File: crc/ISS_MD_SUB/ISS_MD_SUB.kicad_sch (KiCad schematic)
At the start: 3 parts, among them J1 Conn_01x06, SW1 SW_MEC_5E, U1 STM32F303K8Tx

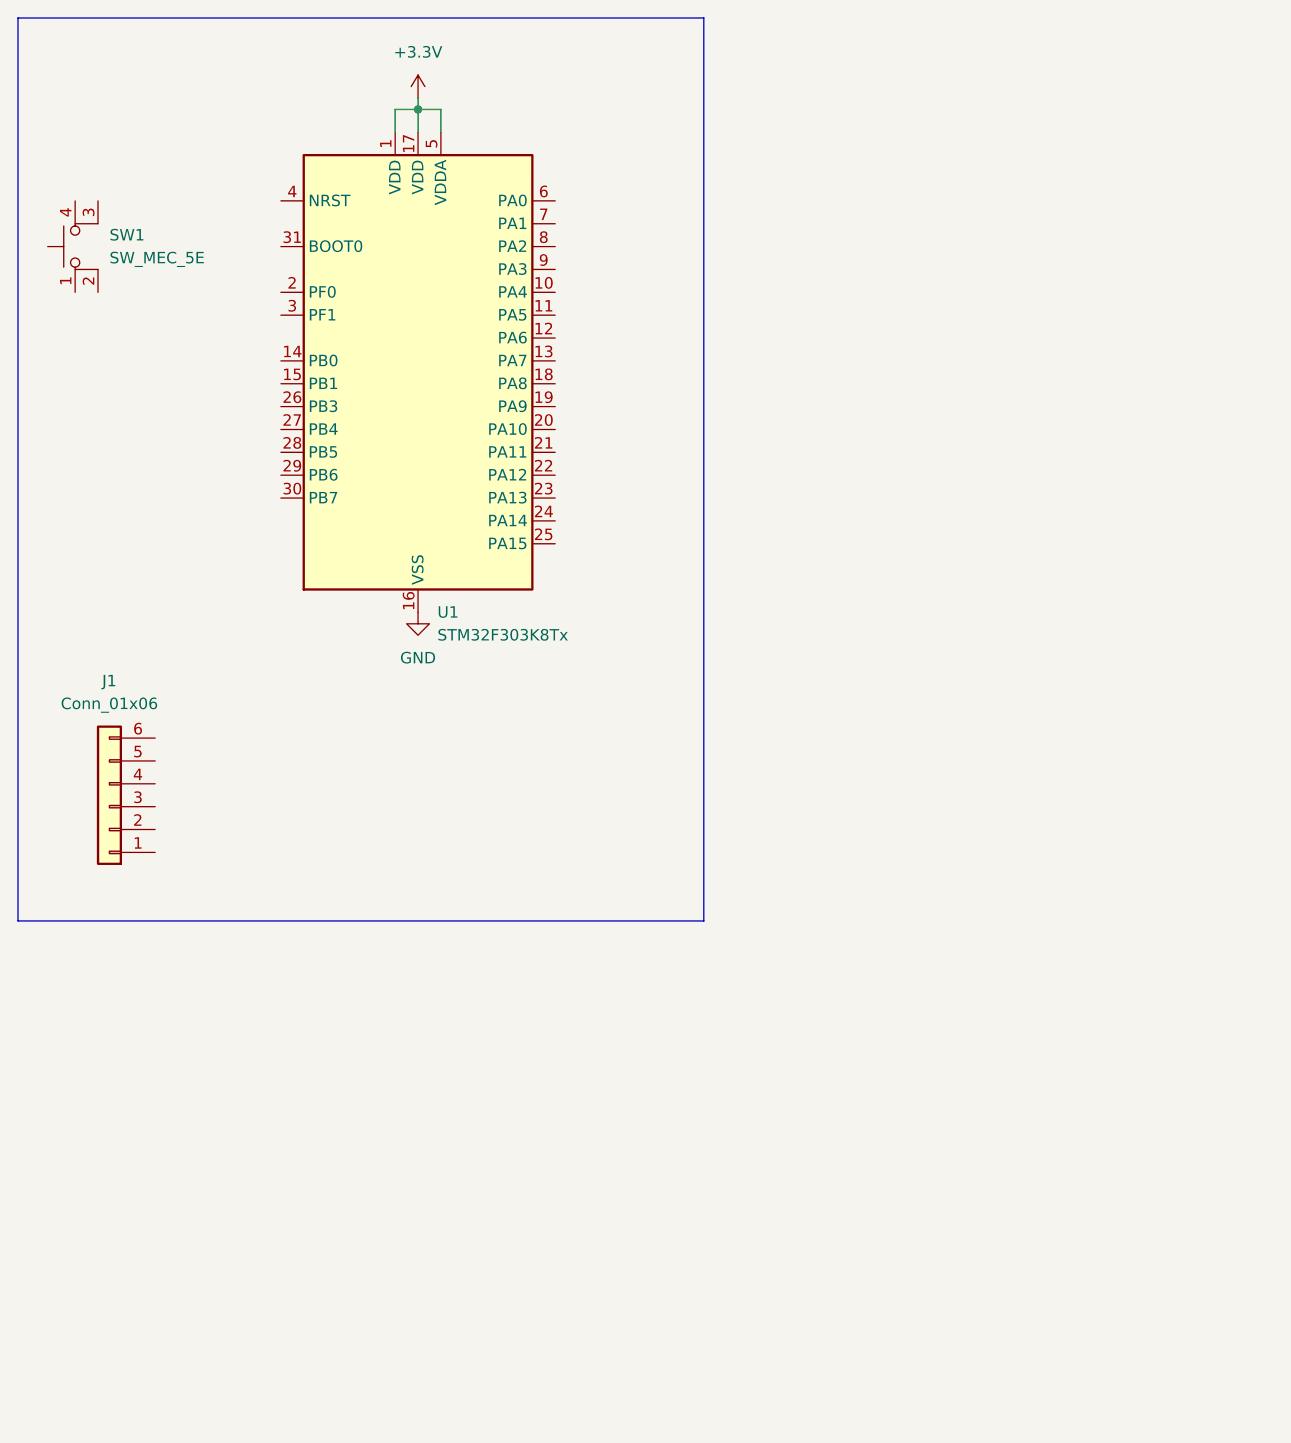
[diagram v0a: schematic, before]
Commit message: 基板2枚め
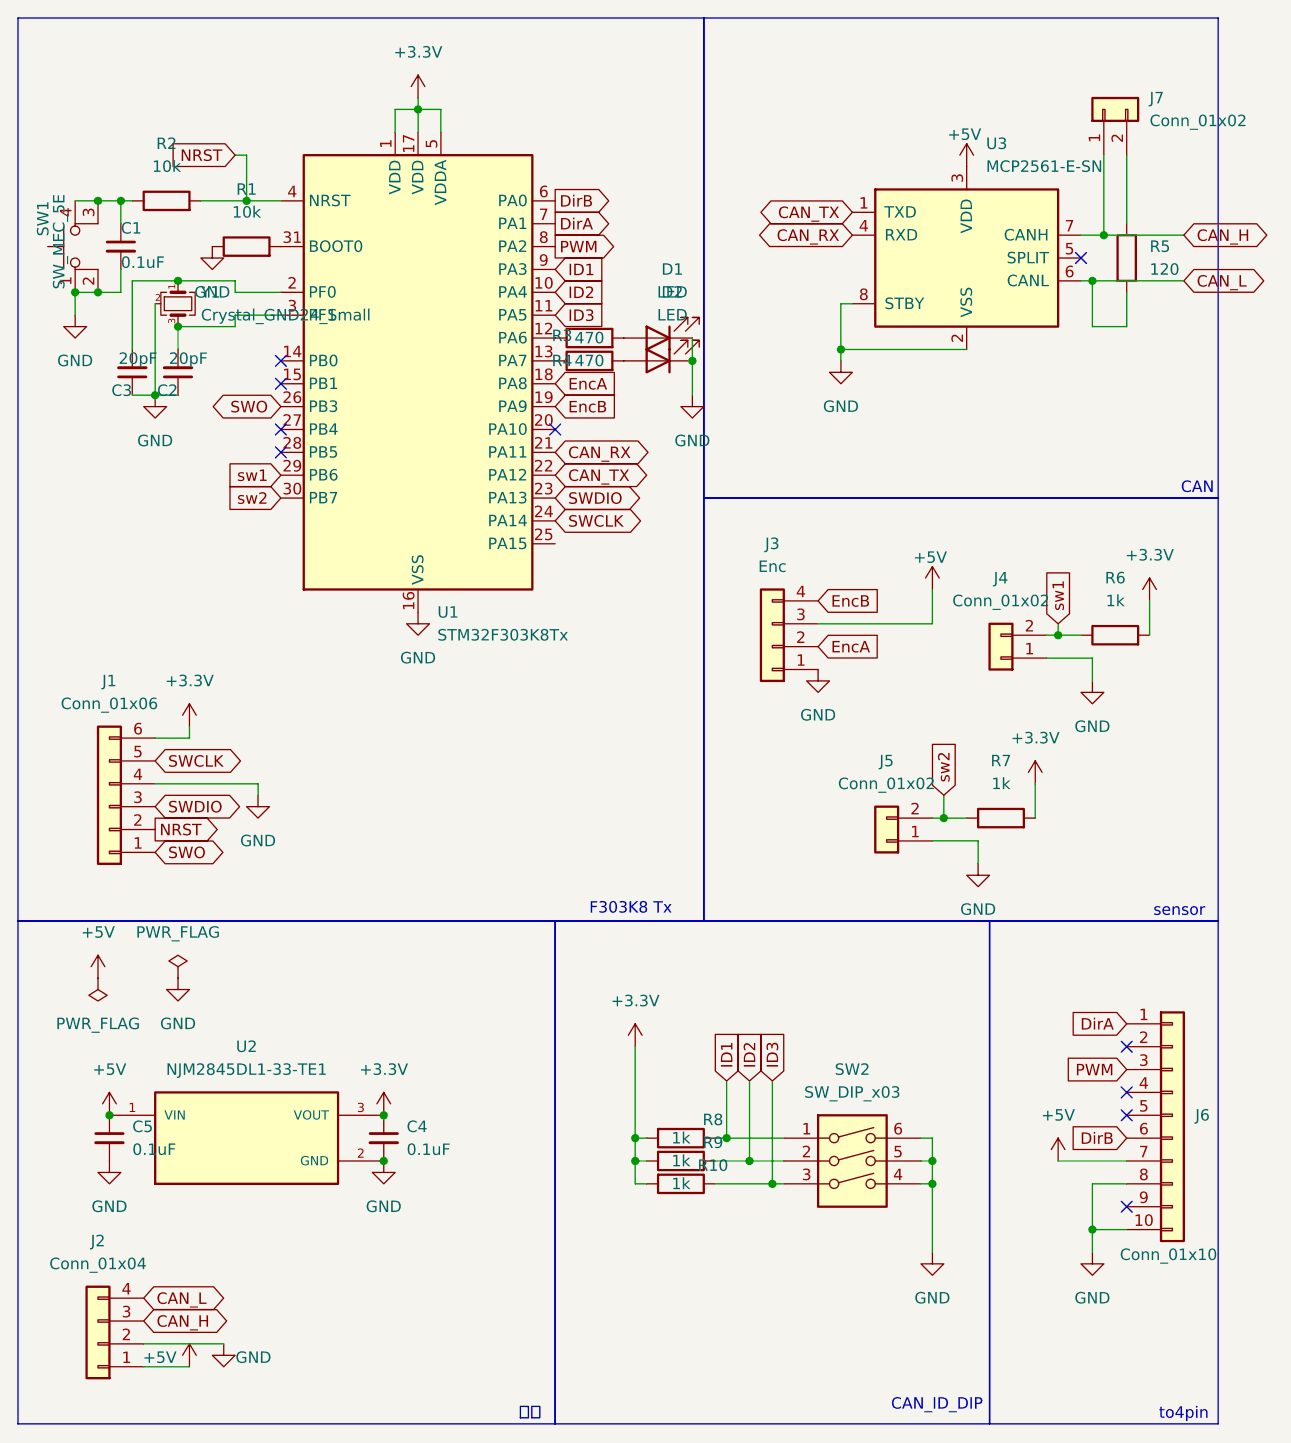
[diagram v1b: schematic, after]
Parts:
- added C1, C4, C5: 0.1uF, Capacitor_SMD:C_0603_1608Metric_Pad1.08x0.95mm_HandSolder, symbol Device:C_Small
- added C2, C3: 20pF, Capacitor_SMD:C_0603_1608Metric_Pad1.08x0.95mm_HandSolder, symbol Device:C_Small
- added D1, D2: LED, LED_SMD:LED_0603_1608Metric_Pad1.05x0.95mm_HandSolder, symbol Device:LED
- added J2: Conn_01x04, Connector_JST:JST_XH_S4B-XH-A_1x04_P2.50mm_Horizontal, symbol Connector_Generic:Conn_01x04
- added J3: Enc, Connector_JST:JST_XH_S4B-XH-A_1x04_P2.50mm_Horizontal, symbol Connector_Generic:Conn_01x04
- added J4, J5: Conn_01x02, Connector_JST:JST_XH_B2B-XH-A_1x02_P2.50mm_Vertical, symbol Connector_Generic:Conn_01x02
- added J6: Conn_01x10, Connector_PinSocket_2.54mm:PinSocket_1x10_P2.54mm_Vertical, symbol Connector_Generic:Conn_01x10
- added J7: Conn_01x02, Connector_PinHeader_2.54mm:PinHeader_1x02_P2.54mm_Vertical, symbol Connector_Generic:Conn_01x02
- added R1, R2: 10k, Resistor_SMD:R_0603_1608Metric_Pad0.98x0.95mm_HandSolder, symbol Device:R
- added R10, R6, R7, R8, R9: 1k, Resistor_SMD:R_0603_1608Metric_Pad0.98x0.95mm_HandSolder, symbol Device:R
- added R3, R4: 470, Resistor_SMD:R_0603_1608Metric_Pad0.98x0.95mm_HandSolder, symbol Device:R
- added R5: 120, Resistor_SMD:R_0603_1608Metric_Pad0.98x0.95mm_HandSolder, symbol Device:R
- added SW2: SW_DIP_x03, Button_Switch_SMD:SW_DIP_SPSTx03_Slide_6.7x9.18mm_W6.73mm_P2.54mm_LowProfile_JPin, symbol Switch:SW_DIP_x03
- added U2: NJM2845DL1-33-TE1, NJM2845DL1-33-TE1:DPAK228P968X238-4N, symbol NJM2845DL1-33-TE1:NJM2845DL1-33-TE1
- added U3: MCP2561-E-SN, Package_SO:SOIC-8_3.9x4.9mm_P1.27mm, symbol Interface_CAN_LIN:MCP2561-E-SN
- added Y1: Crystal_GND24_Small, TSX_3225_25_0000MF10P_C0:XTAL_TSX-3225_25.0000MF10P-C0, symbol Device:Crystal_GND24_Small
- J1: footprint (none) -> Connector_PinHeader_2.54mm:PinHeader_1x06_P2.54mm_Vertical
- SW1: footprint (none) -> SKRPABE010:SW4_SKRPABE010_ALPS
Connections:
- net +3.3V: now also J1.6 (Pin_6), C4.1, R10.2, R6.2, R7.2, R8.2, R9.2, U2.3 (VOUT)
- net GND: now also J1.4 (Pin_4), SW1.1, SW1.2, C1.2, C2.1, C3.1, C4.2, C5.2, D1.1 (K), D2.1 (K), J2.2 (Pin_2), J3.1 (Pin_1), J4.1 (Pin_1), J5.1 (Pin_1), J6.10 (Pin_10), J6.8 (Pin_8), R1.1, SW2.4, SW2.5, SW2.6, U2.2 (GND), U3.2 (VSS), U3.8 (STBY), Y1.2 (G), Y1.4 (G)
- net SWO: now reaches J1.1 (Pin_1)
- net SWO: now also U1.26 (PB3)
- net NRST: now reaches J1.2 (Pin_2)
- net NRST: now also U1.4 (NRST), R2.2
- net SWDIO: now reaches J1.3 (Pin_3)
- net SWDIO: now also U1.23 (PA13)
- net SWCLK: now reaches J1.5 (Pin_5)
- net SWCLK: now also U1.24 (PA14)
- net at SW1.3 (K): now also SW1.4 (A), C1.1, R2.1
- net ID2: now reaches U1.10 (PA4)
- net ID2: now also R9.1, SW2.2
- net ID3: now reaches U1.11 (PA5)
- net ID3: now also R10.1, SW2.3
- net at U1.12 (PA6): now also R3.1
- net at U1.13 (PA7): now also R4.1
- net EncA: now reaches U1.18 (PA8)
- net EncA: now also J3.2 (Pin_2)
- net EncB: now reaches U1.19 (PA9)
- net EncB: now also J3.4 (Pin_4)
- net at U1.2 (PF0): now also C3.2, Y1.1
- net CAN_RX: now reaches U1.21 (PA11)
- net CAN_RX: now also U3.4 (RXD)
- net CAN_TX: now reaches U1.22 (PA12)
- net CAN_TX: now also U3.1 (TXD)
- net sw1: now reaches U1.29 (PB6)
- net sw1: now also J4.2 (Pin_2), R6.1
- net at U1.3 (PF1): now also C2.2, Y1.3
- net sw2: now reaches U1.30 (PB7)
- net sw2: now also J5.2 (Pin_2), R7.1
- net at U1.31 (BOOT0): now also R1.2
- net DirB: now reaches U1.6 (PA0)
- net DirB: now also J6.6 (Pin_6)
- net DirA: now reaches U1.7 (PA1)
- net DirA: now also J6.1 (Pin_1)
- net PWM: now reaches U1.8 (PA2)
- net PWM: now also J6.3 (Pin_3)
- net ID1: now reaches U1.9 (PA3)
- net ID1: now also R8.1, SW2.1
- new net: D1.2 (A), R3.2
- new net: D2.2 (A), R4.2
- new net: J7.2 (Pin_2), R5.1
- new net +5V: C5.1, J2.1 (Pin_1), J3.3 (Pin_3), J6.7 (Pin_7), U2.1 (VIN), U3.3 (VDD)
- new net CAN_H: J2.3 (Pin_3), J7.1 (Pin_1), U3.7 (CANH)
- new net CAN_L: J2.4 (Pin_4), R5.2, U3.6 (CANL)
- no-connect marks 0 -> 10
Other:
- note added: "CAN"
- note added: "CAN_ID_DIP"
- note added: "F303K8 Tx"
- note added: "sensor"
- note added: "to4pin"
- note added: "電源"

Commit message: ノード完成
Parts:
- SW2: footprint Button_Switch_SMD:SW_DIP_SPSTx03_Slide_6.7x9.18mm_W6.73mm_P2.54mm_LowProfile_JPin -> Button_Switch_THT:SW_DIP_SPSTx03_Slide_9.78x9.8mm_W7.62mm_P2.54mm
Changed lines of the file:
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@@
 			)
 		)
-		(property "Footprint" "Button_Switch_SMD:SW_DIP_SPSTx03_Slide_6.7x9.18mm_W6.73mm_P2.54mm_LowProfile_JPin"
+		(property "Footprint" "Button_Switch_THT:SW_DIP_SPSTx03_Slide_9.78x9.8mm_W7.62mm_P2.54mm"
 			(at 105.41 142.24 0)
 			(hide yes)
